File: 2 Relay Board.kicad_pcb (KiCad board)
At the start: 2 copper layers, 158 x 75 mm, 45 parts, among them J1 Conn_01x02, J2 Conn_01x03, J3 Conn_01x05, K1 RAYEX-L90, K2 RAYEX-L90, Q1 BD139, Q2 BD139, U1 N76E003, U3 LM7809_TO220, U4 AMS1117-5.0, U5 CA56-12EWA, U6 CA56-12EWA

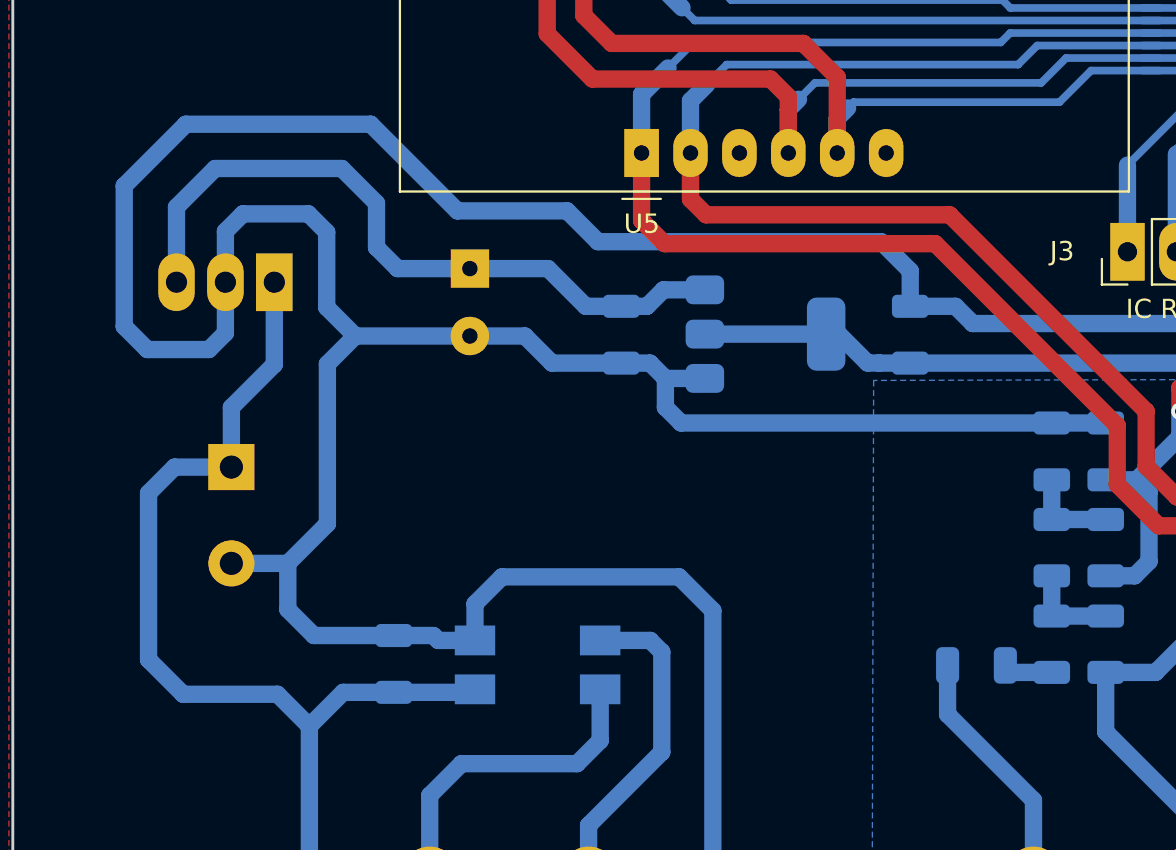
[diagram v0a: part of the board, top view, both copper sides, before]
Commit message: this version hase small 7805 v1.1
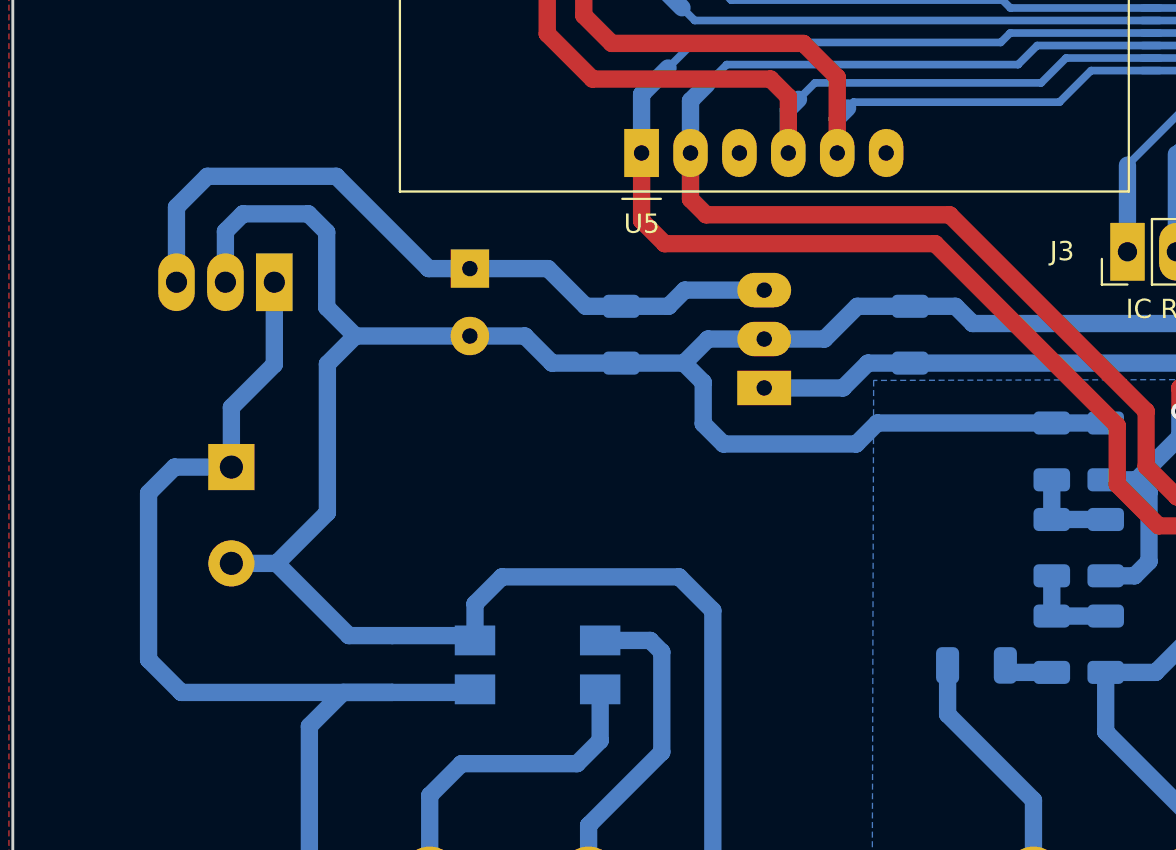
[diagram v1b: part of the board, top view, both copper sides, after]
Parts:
- removed C3: 0.1uf/50v, My Custom Footprint:C_1206_3216Metric
- removed U4: AMS1117-5.0, Package_TO_SOT_SMD:SOT-223-3_TabPin2
- added U2: LM2936-5.0_TO92, My Custom Footprint:TO-92_Inline_Wide_LM78L05, B.Cu at (110.8, 101.6)
- C1, C12, C2, C6, C8: value 10uf/50v -> C
- C10, C5, C7: value 0.1uf/50v -> C
- U3: value LM7809_TO220 -> LM7812_TO220
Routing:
- net VSS: track 370.5 -> 318.0 mm
- net +24V: track 273.8 -> 277.2 mm
- net VDD: track 50.8 -> 47.6 mm
- net +12V: track 36.8 -> 38.2 mm
